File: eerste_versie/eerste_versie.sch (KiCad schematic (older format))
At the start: 19 parts, among them J1 105017-1001, J2 Conn_01x02, SW1 SW_DPDT_x2, U1 ESP32-WROOM-32U, U2 AMS1117-3.3

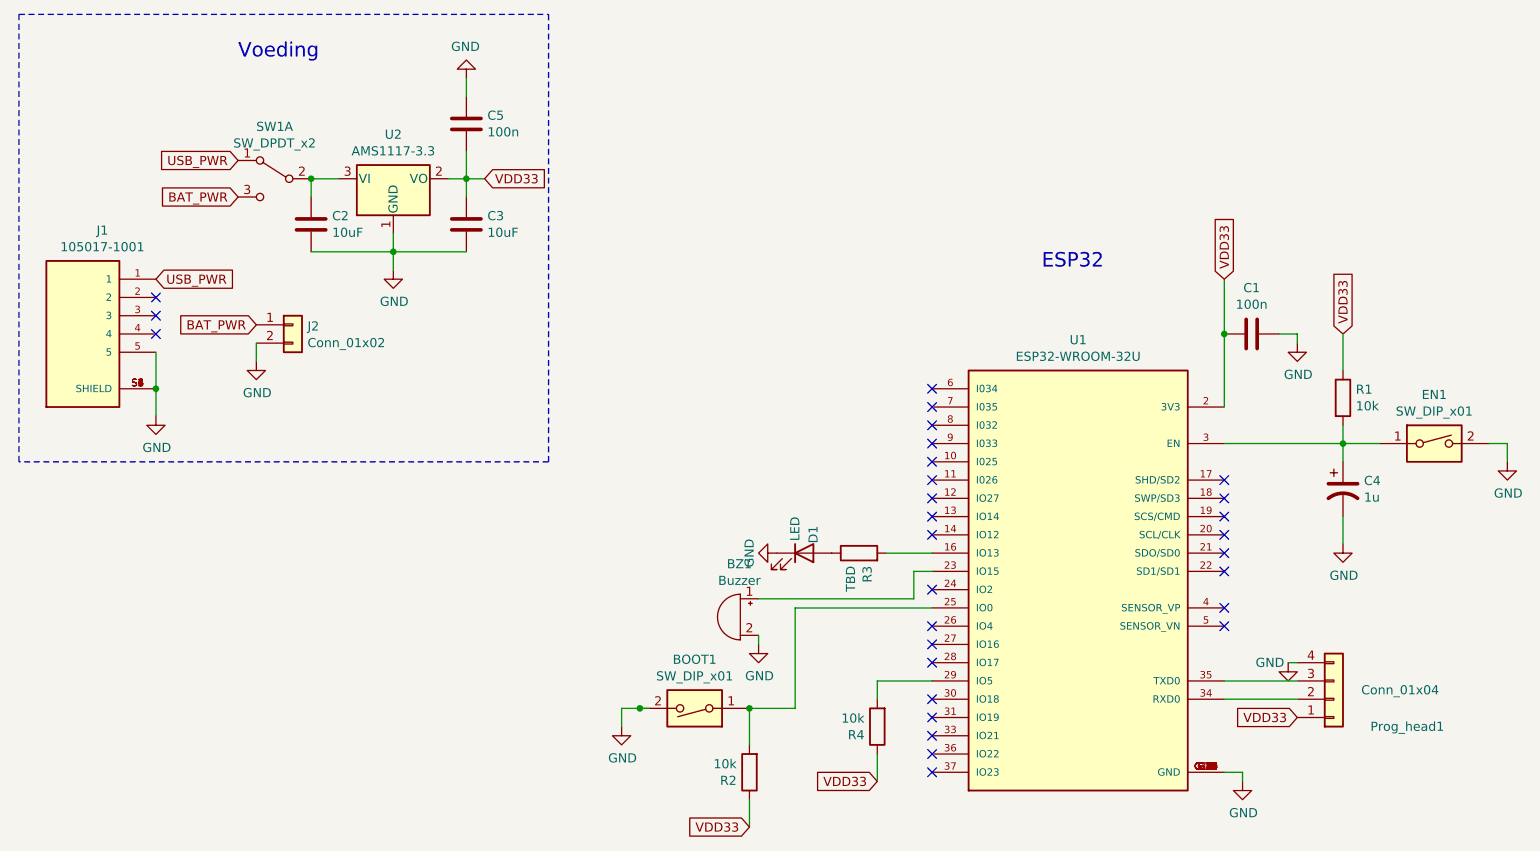
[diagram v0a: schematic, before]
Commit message: opgemaakte versie voor github verslag
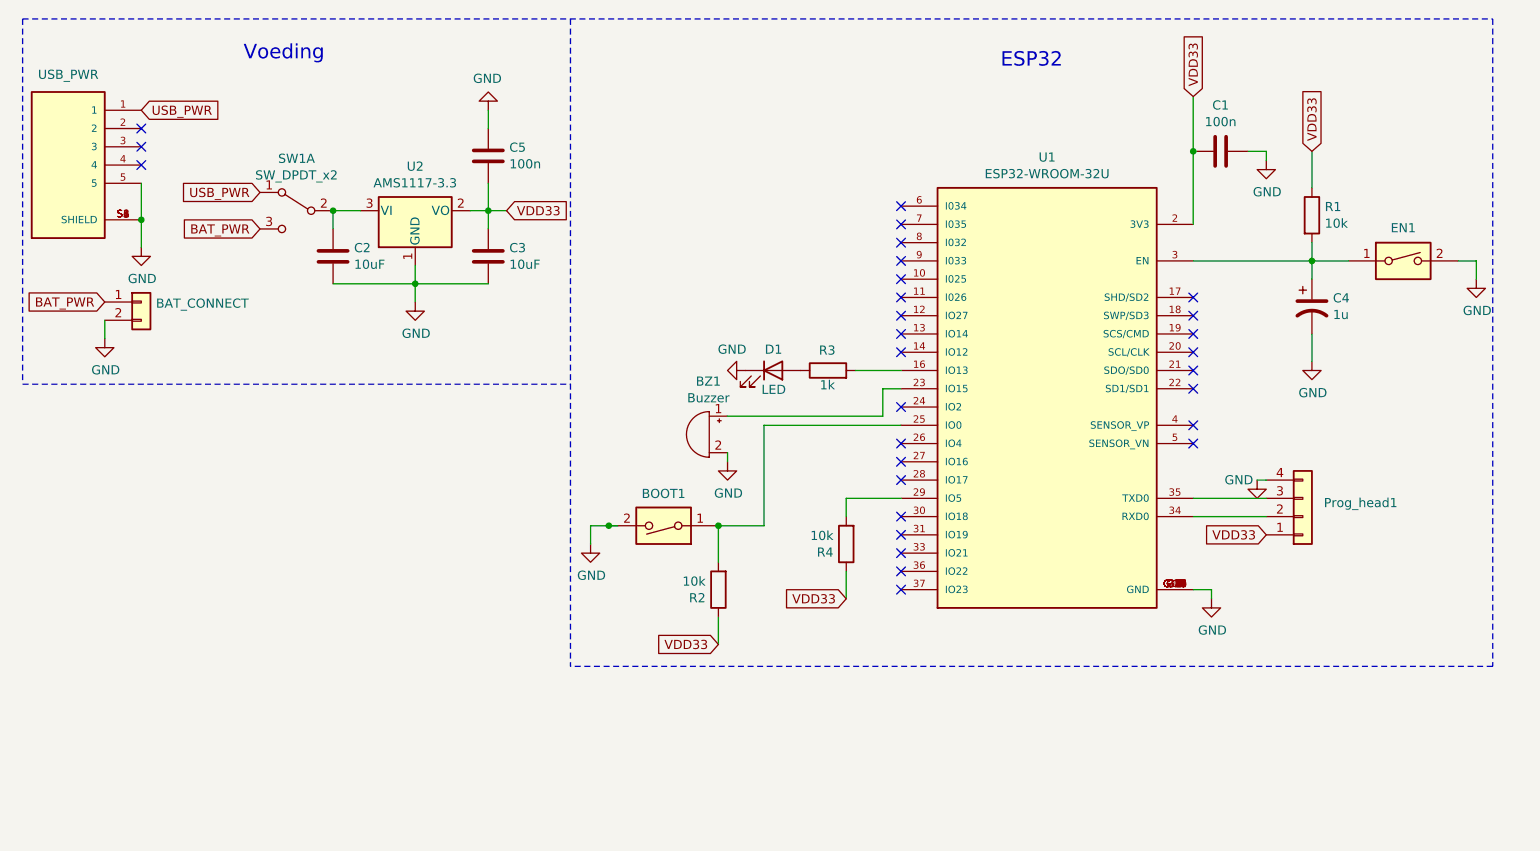
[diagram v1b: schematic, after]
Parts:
- R3: value TBD -> 1k
- renumbered J2 to BAT_CONNECT, J1 to USB_PWR
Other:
- moved on the sheet: BAT_CONNECT, BOOT1, BZ1, C1, C2, C3, C4, C5, D1, EN1, Prog_head1, R1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
